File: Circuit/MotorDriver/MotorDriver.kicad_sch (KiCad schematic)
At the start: 25 parts, among them J3 Conn_01x03_Pin, J4 Conn_01x04_Pin, J5 Conn_01x06_Pin, J6 Conn_01x02_Pin, U3 DRV8316RRGFR, U4 XC6206PxxxMR

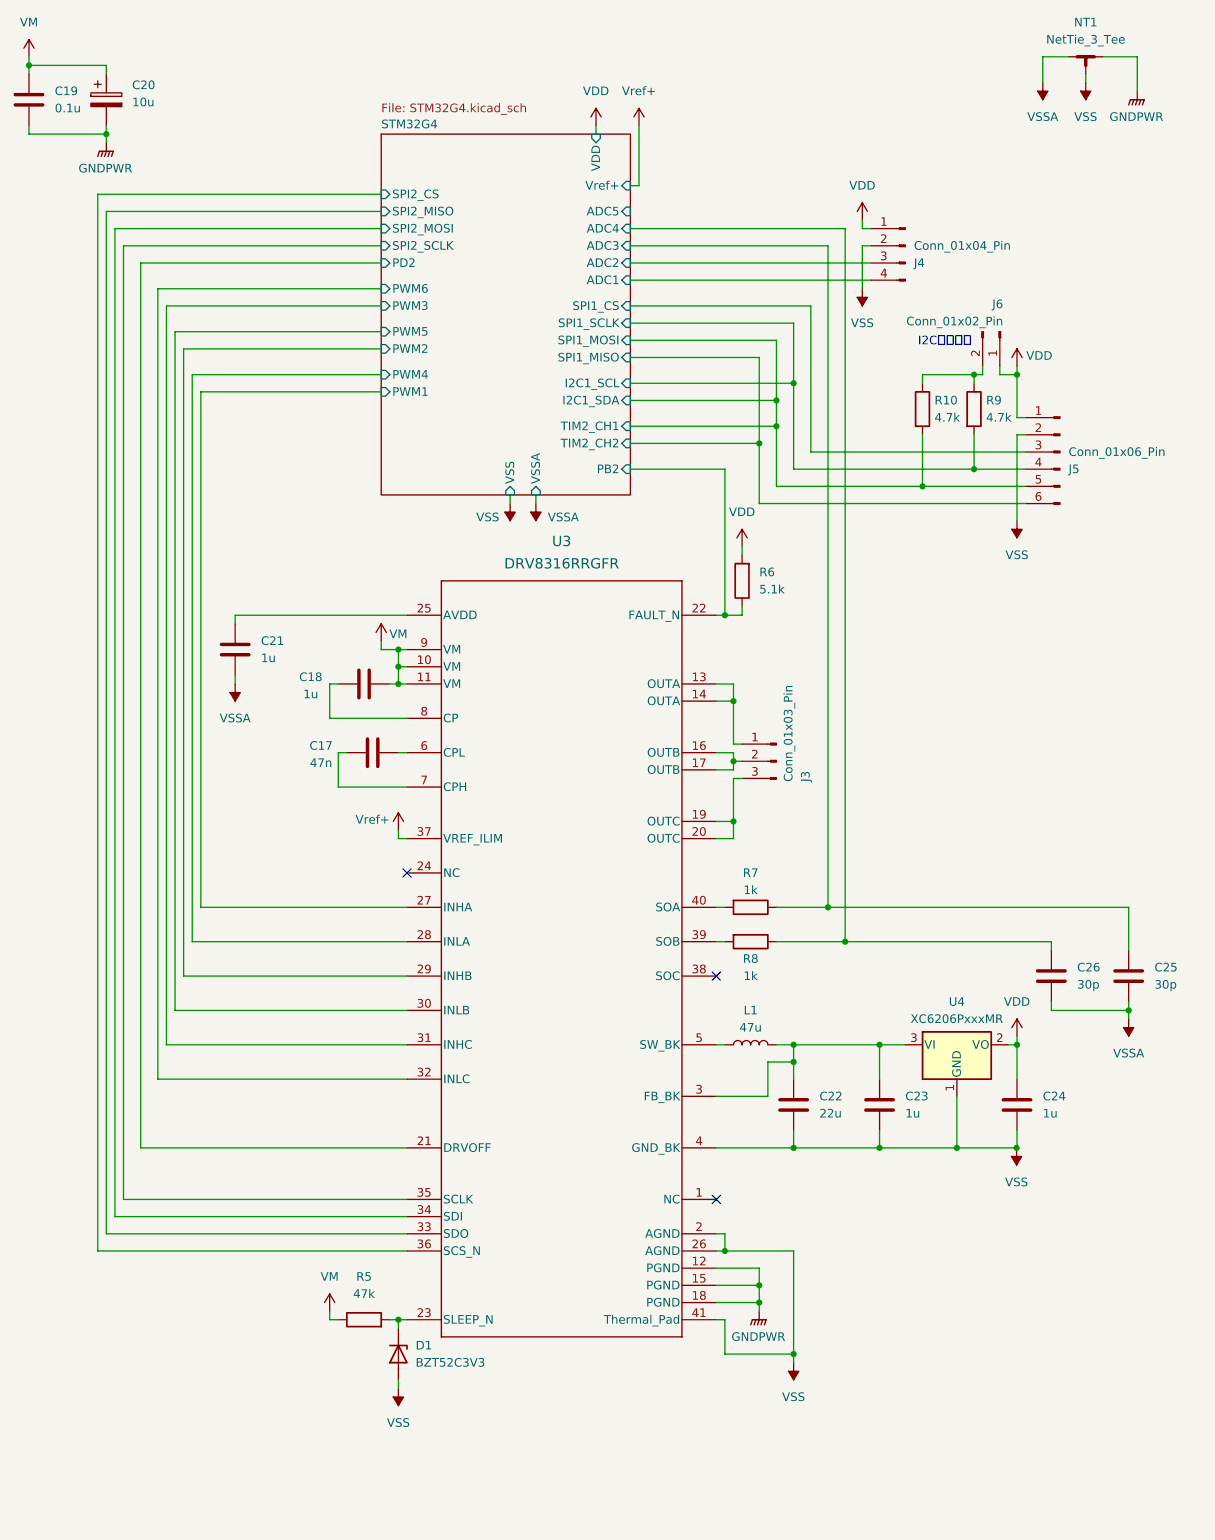
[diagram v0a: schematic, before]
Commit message: 回路図完成
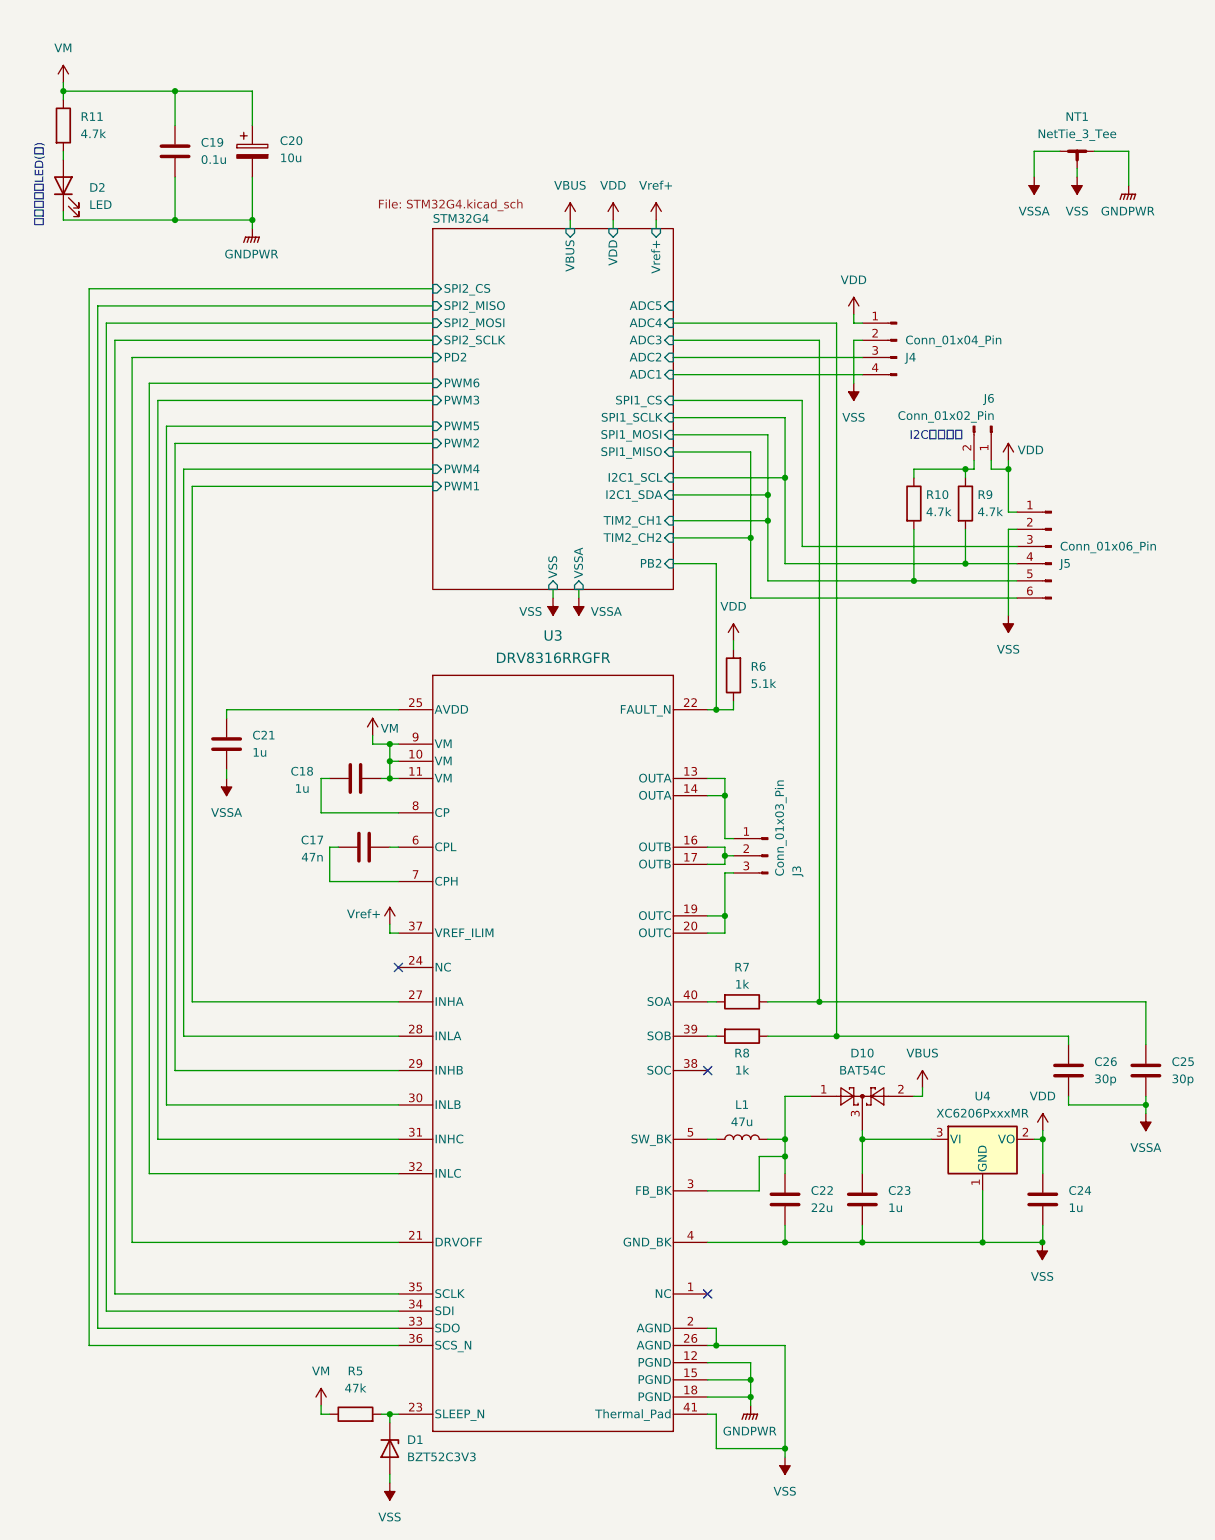
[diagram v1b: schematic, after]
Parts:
- added D10: BAT54C, Package_TO_SOT_SMD:SOT-23, symbol Diode:BAT54C
- added D2: LED, symbol Device:LED
- added R11: 4.7k, Resistor_SMD:R_1206_3216Metric, symbol Device:R
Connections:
- net GNDPWR: now also D2.1 (K)
- net VM: now also R11.1
- net at C22.1, L1.2, U3.3 (FB_BK): now also D10.1; no longer C23.1, U4.3 (VI)
- new net: D2.2 (A), R11.2
- new net: C23.1, D10.3, U4.3 (VI)
- new net VBUS: D10.2
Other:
- sheet STM32G4 ports: added VBUS; removed none
- note added: "モータ電源LED(緑)"
- moved on the sheet: C17, C18, C19, C20, C21, C22, C23, C24, C25, C26, D1, J3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
